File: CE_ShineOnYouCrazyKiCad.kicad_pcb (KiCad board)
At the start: 2 copper layers, 5 parts, among them J1 CONN_02X05

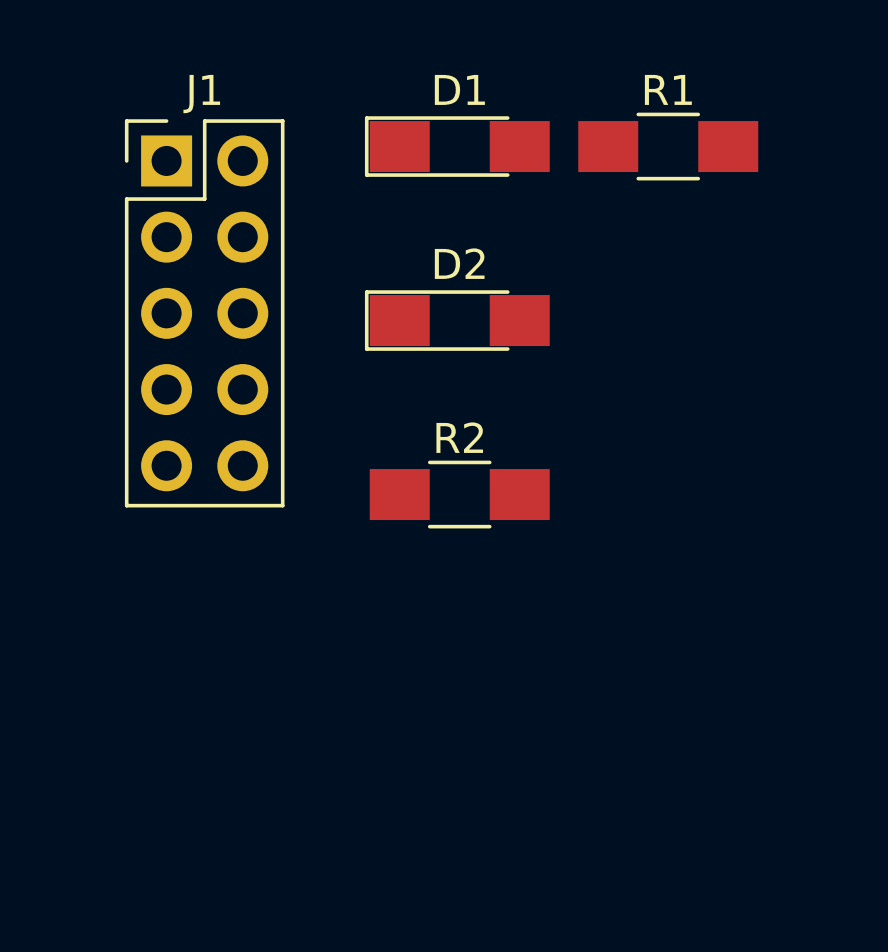
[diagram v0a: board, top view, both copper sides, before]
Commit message: Completed PCB
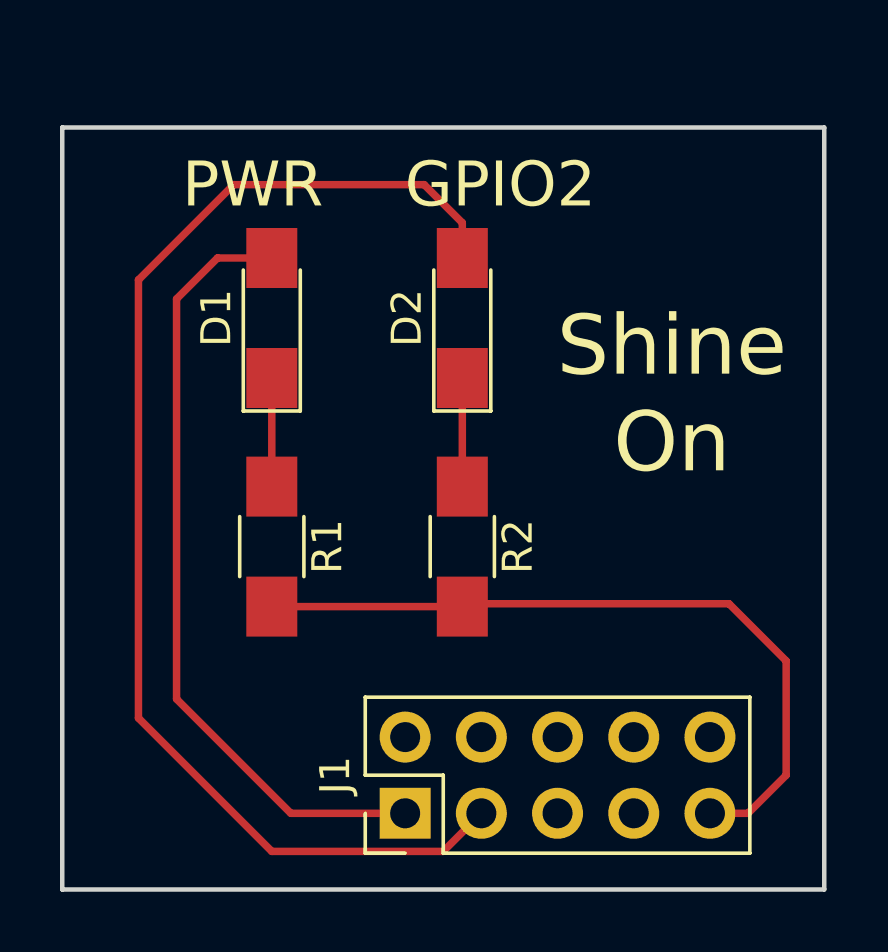
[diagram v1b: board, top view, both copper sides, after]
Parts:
- moved J1 23.2 mm to (161.3, 133.3), turned to 90 degrees
- moved R1 18.8 mm to (156.8, 124.5), turned to 270 degrees
- moved D1 8.48 mm to (156.8, 116.8), turned to 90 degrees
- moved R2 1.74 mm to (163.2, 124.5), turned to 270 degrees
- moved D2 0.12 mm to (163.2, 116.8), turned to 90 degrees
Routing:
- net Net-(D2-Pad2): track 0.00 -> 42.2 mm
- net Net-(D1-Pad2): track 0.00 -> 26.3 mm
- net Net-(J1-Pad9): track 0.00 -> 24.8 mm
- net Net-(D2-Pad1): track 0.00 -> 3.62 mm
- net Net-(D1-Pad1): track 0.00 -> 3.62 mm
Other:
- board outline added: 25.4 x 25.4 mm
- board text added: "GPIO2"
- board text added: "PWR"
- board text added: "Shine On"
